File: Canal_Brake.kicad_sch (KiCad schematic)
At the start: 0 parts

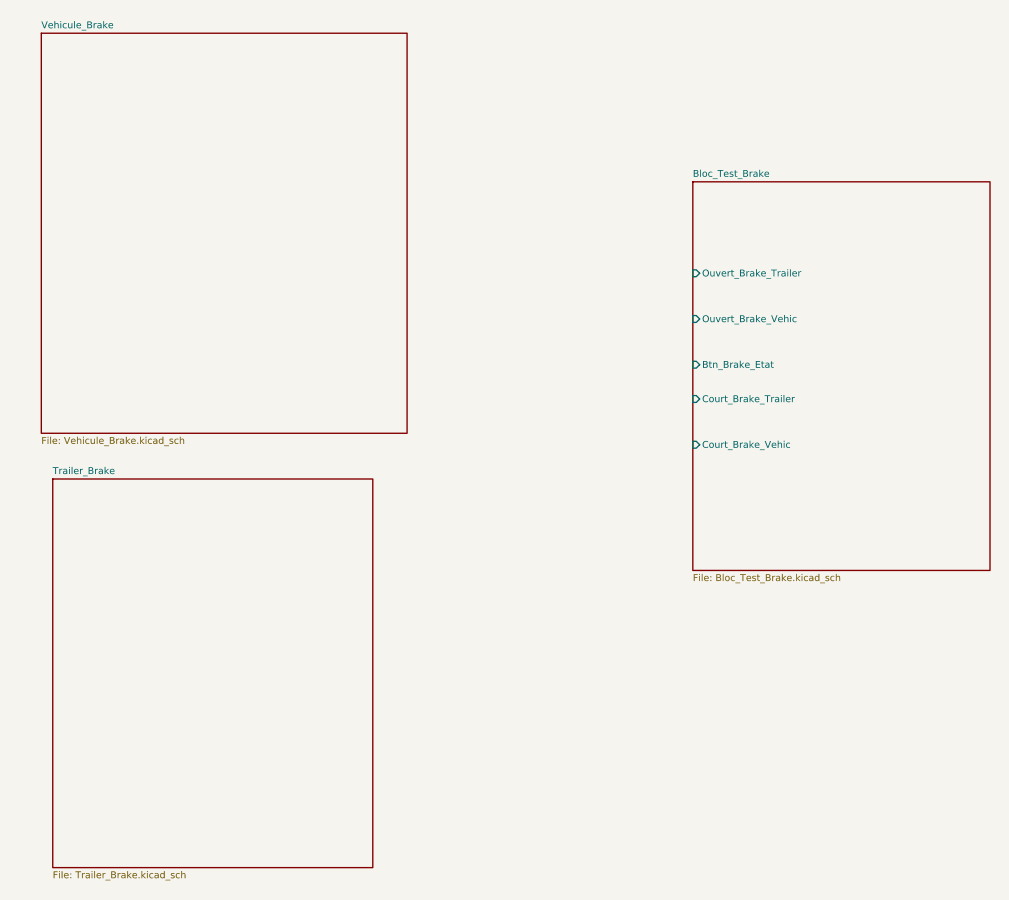
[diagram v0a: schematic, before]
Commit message: Add files via upload
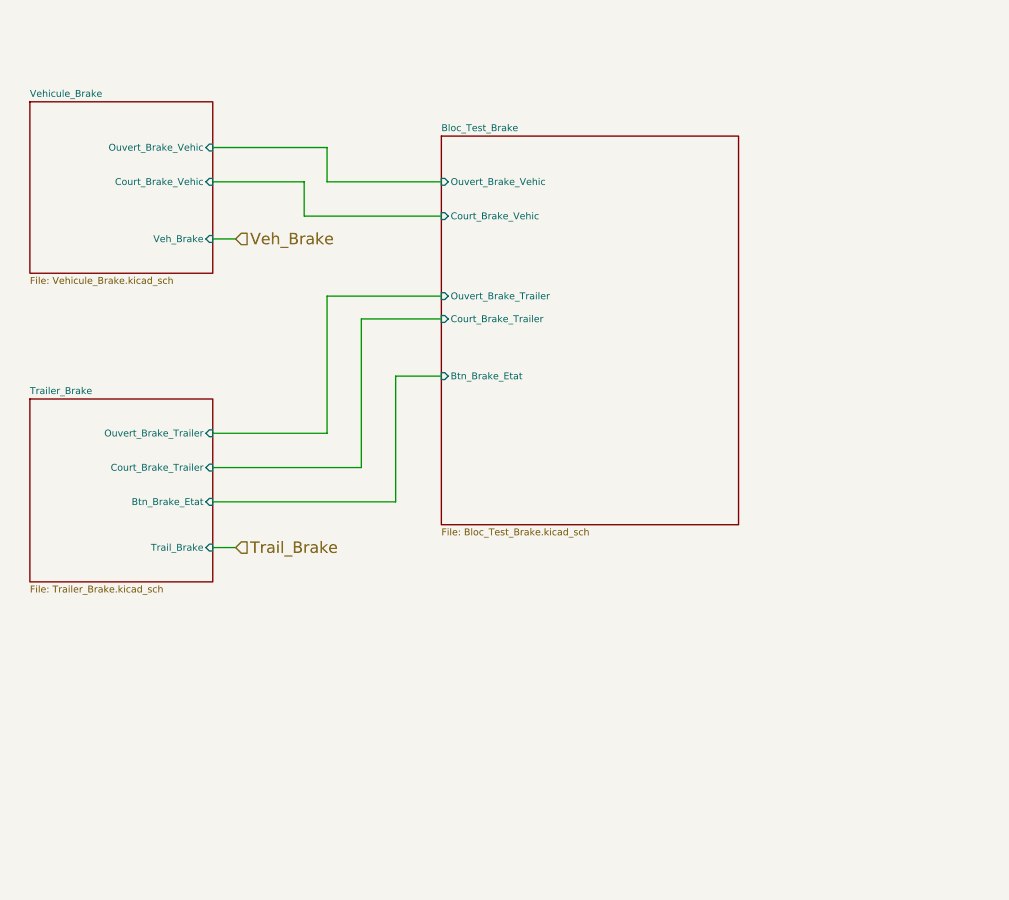
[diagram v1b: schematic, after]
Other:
- sheet Trailer_Brake ports: added Btn_Brake_Etat, Court_Brake_Trailer, Ouvert_Brake_Trailer, Trail_Brake; removed none
- sheet Vehicule_Brake ports: added Court_Brake_Vehic, Ouvert_Brake_Vehic, Veh_Brake; removed none

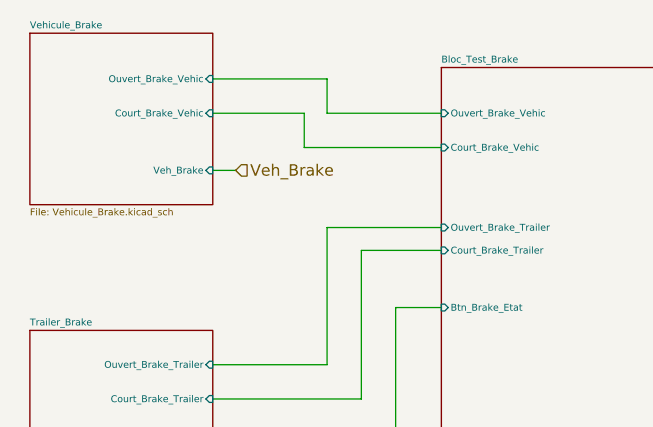
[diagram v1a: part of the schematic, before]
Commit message: Add files via upload
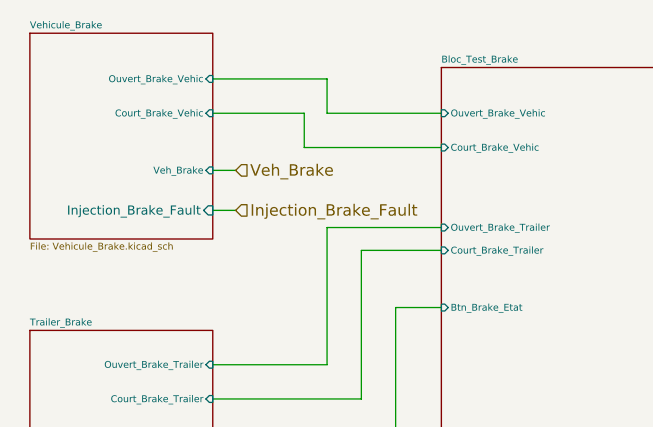
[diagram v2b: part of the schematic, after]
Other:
- sheet Vehicule_Brake ports: added Injection_Brake_Fault; removed none
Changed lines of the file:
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@@
+	(wire
+		(pts
+			(xy 38.1 40.005) (xy 40.64 40.005)
+		)
+		(stroke
+			(width 0)
+			(type default)
+		)
+	)
 	(wire
 		(pts
@@
 		)
 	)
+	(hierarchical_label "Injection_Brake_Fault"
+		(shape input)
+		(at 40.64 40.005 0)
+		(effects
+			(font
+				(size 1.27 1.27)
+			)
+			(justify left)
+		)
+	)
 	(hierarchical_label "Trail_Brake"
 		(shape input)
@@
 	(sheet
 		(at 17.78 20.32)
-		(size 20.32 19.05)
+		(size 20.32 22.86)
 		(exclude_from_sim no)
 		(in_bom yes)
@@
 		)
 		(property "Sheetfile" "Vehicule_Brake.kicad_sch"
-			(at 17.78 39.7514 0)
+			(at 17.78 43.5614 0)
 			(show_name no)
 			(do_not_autoplace no)
@@
 				)
 				(justify right)
+			)
+		)
+		(pin "Injection_Brake_Fault" input
+			(at 38.1 40.005 0)
+			(effects
+				(font
+					(size 1.016 1.016)
+				)
+				(justify right)

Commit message: Add files via upload
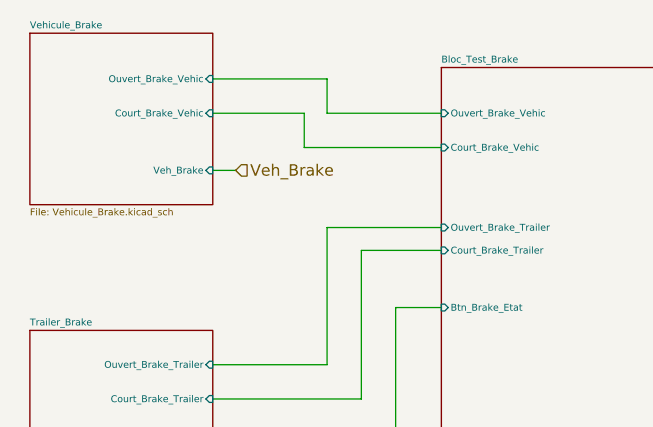
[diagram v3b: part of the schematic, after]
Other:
- sheet Vehicule_Brake ports: added none; removed Injection_Brake_Fault
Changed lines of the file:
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@@
-	(wire
-		(pts
-			(xy 38.1 40.005) (xy 40.64 40.005)
-		)
-		(stroke
-			(width 0)
-			(type default)
-		)
-	)
 	(wire
 		(pts
@@
 		)
 	)
-	(hierarchical_label "Injection_Brake_Fault"
-		(shape input)
-		(at 40.64 40.005 0)
-		(effects
-			(font
-				(size 1.27 1.27)
-			)
-			(justify left)
-		)
-	)
 	(hierarchical_label "Trail_Brake"
 		(shape input)
@@
 	(sheet
 		(at 17.78 20.32)
-		(size 20.32 22.86)
+		(size 20.32 19.05)
 		(exclude_from_sim no)
 		(in_bom yes)
@@
 		)
 		(property "Sheetfile" "Vehicule_Brake.kicad_sch"
-			(at 17.78 43.5614 0)
+			(at 17.78 39.7514 0)
 			(show_name no)
 			(do_not_autoplace no)
@@
 				)
 				(justify right)
-			)
-		)
-		(pin "Injection_Brake_Fault" input
-			(at 38.1 40.005 0)
-			(effects
-				(font
-					(size 1.016 1.016)
-				)
-				(justify right)
